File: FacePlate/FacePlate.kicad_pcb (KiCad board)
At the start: 4 copper layers, 131.1 x 44 mm, 76 parts, among them J2 GPIO, J3 Conn_01x04_Pin, U4 SX1280, U5 MCP2515-xST, U6 MCP2551-I-SN, U7 AMS1117-3.3, Y2 ABM3-8.000MHZ-D2Y-T

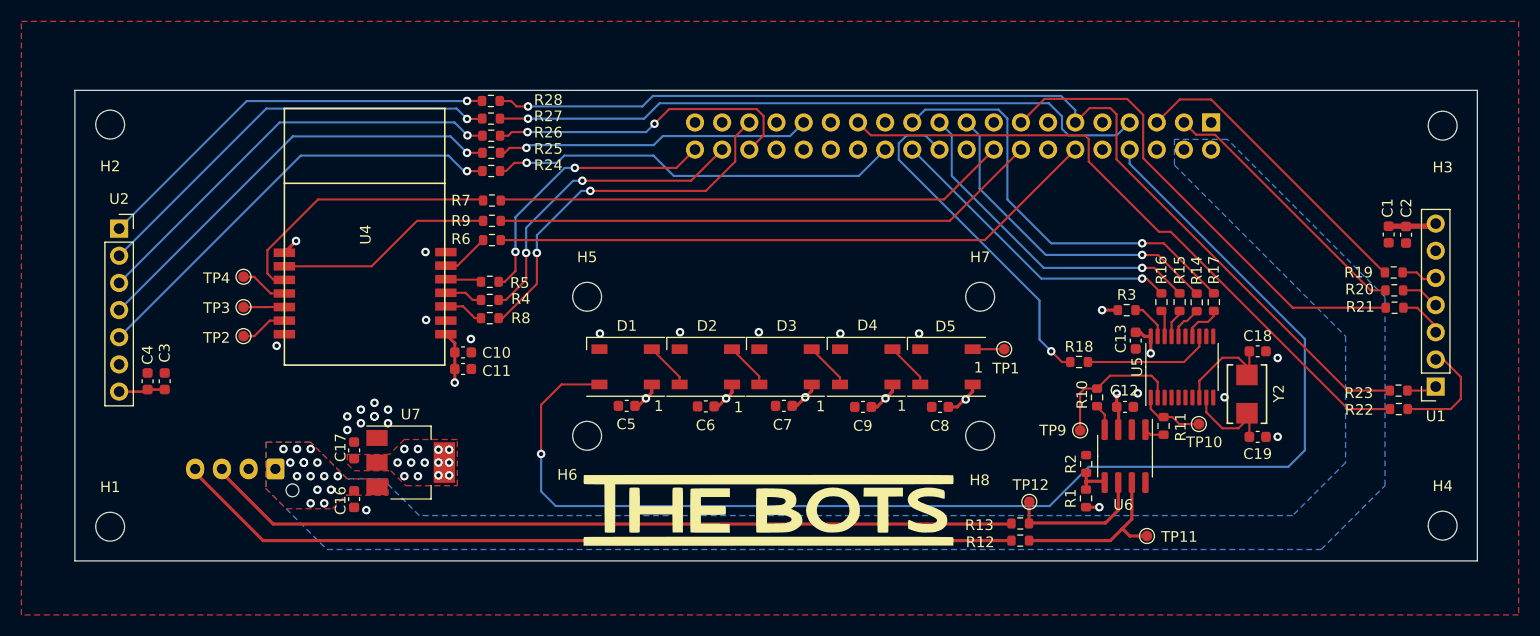
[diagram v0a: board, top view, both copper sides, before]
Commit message: faceplate updates
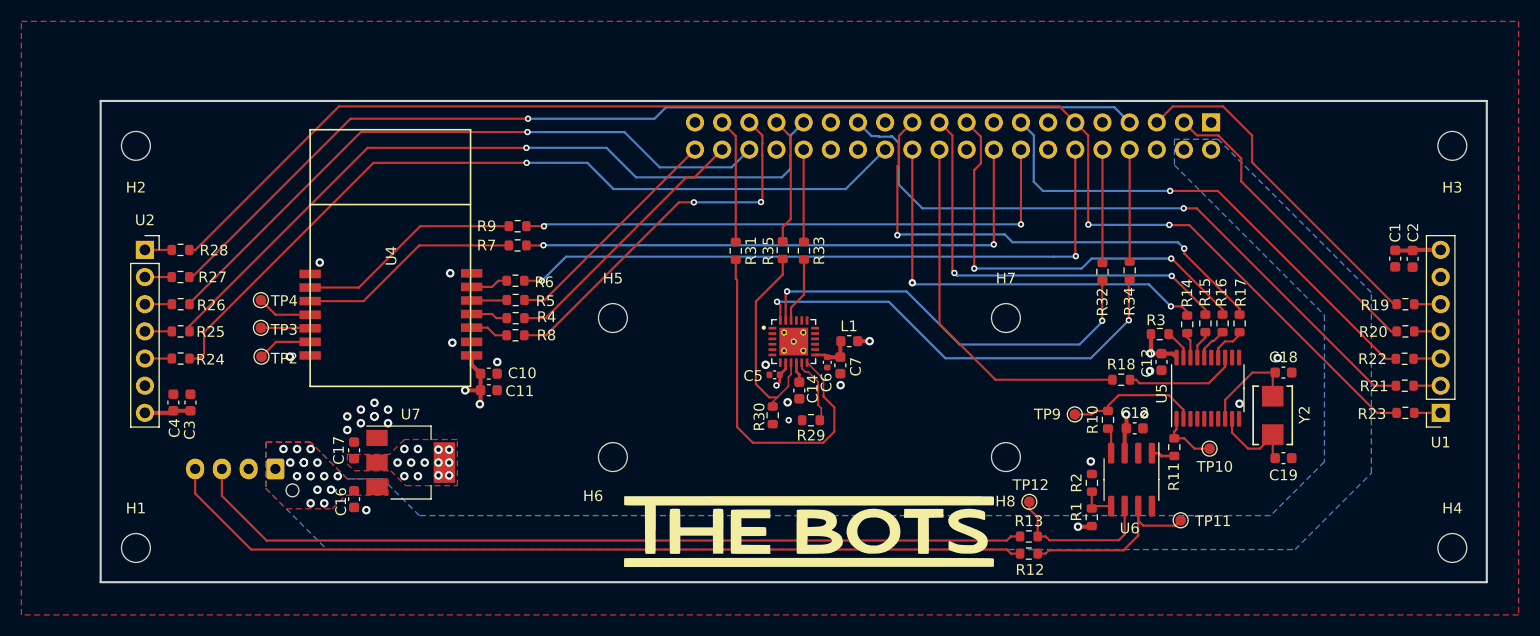
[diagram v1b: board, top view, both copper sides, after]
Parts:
- removed C8, C9: 100n, Capacitor_SMD:C_0603_1608Metric
- removed D1, D2, D3, D4, D5: WS2812B, LED_SMD:LED_WS2812B_PLCC4_5.0x5.0mm_P3.2mm
- removed TP1: TestPoint, TestPoint:TestPoint_Pad_D1.0mm
- added C14: 10u, bots:C_0603_1608Metric, F.Cu at (167.7, 84.1)
- added L1: 120R, bots:L_0603_1608Metric, F.Cu at (172.4, 79.5)
- added R29: 10k, bots:R_0603_1608Metric, F.Cu at (168.8, 86.8)
- added R30: 10k, bots:R_0603_1608Metric, F.Cu at (165.3, 86.4)
- added R31: 0R, bots:R_0603_1608Metric, F.Cu at (161.8, 71.0)
- added R32: 0R, bots:R_0603_1608Metric, F.Cu at (196.1, 73.0)
- added R33: 0R, bots:R_0603_1608Metric, F.Cu at (168.2, 71.0)
- added R34: 0R, bots:R_0603_1608Metric, F.Cu at (198.6, 72.8)
- added R35: 0R, bots:R_0603_1608Metric, F.Cu at (166.2, 70.9)
- added U3: ICM-20689, bots:QFN50P400X400X95-24N, F.Cu at (167.2, 79.5)
- C1, C10, C11, C2, C3, C4: value 100n -> 0.1u; footprint Capacitor_SMD:C_0603_1608Metric -> bots:C_0603_1608Metric
- C12, C13, C16: footprint Capacitor_SMD:C_0603_1608Metric -> bots:C_0603_1608Metric
- C17: value 22u -> 10u; footprint Capacitor_SMD:C_0603_1608Metric -> bots:C_0603_1608Metric
- C5, C6: footprint Capacitor_SMD:C_0603_1608Metric -> bots:C_0402_1005Metric
- C7: value 100n -> 10u; footprint Capacitor_SMD:C_0603_1608Metric -> bots:C_0603_1608Metric
- R10, R11, R12, R13, R14, R15, R16, R17, R18, R19, R20, R21, R22, R23, R24, R25, R26, R27, R28: value 0k -> 0R; footprint Resistor_SMD:R_0603_1608Metric -> bots:R_0603_1608Metric
- U1, U2: footprint Connector_PinSocket_2.54mm:PinSocket_1x07_P2.54mm_Vertical -> bots:GC9A_Display
- moved R24 33.9 mm to (109.9, 81.1)
- moved R25 33.5 mm to (109.9, 78.5)
- moved R26 33.0 mm to (109.9, 76.0)
- moved R27 32.6 mm to (109.9, 73.5)
- moved R28 32.2 mm to (109.9, 70.9)
- moved C5 14.1 mm to (165.4, 82.6)
- moved C6 12.1 mm to (170.4, 81.4), turned to -90 degrees
- moved R21 7.35 mm to (224.4, 83.6)
- moved C7 6.49 mm to (171.6, 81.7), turned to -90 degrees
- moved R16 6.05 mm to (207.3, 77.8)
- moved R7 4.84 mm to (141.4, 70.5)
- moved R22 4.73 mm to (224.3, 81.1)
- moved R6 4.39 mm to (141.2, 73.8)
- moved R18 4.28 mm to (197.8, 83.1)
- moved G*** 4.27 mm to (168.6, 97.2)
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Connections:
- C6 pad 1: +3.3V -> /IMU/3v3
- C7 pad 1: +3.3V -> /IMU/3v3
- R14 pad 1: Net-(U5-SI) -> Net-(U5-~{CS})
- R14 pad 2: /SPI0_MOSI -> /SPI0_NSS
- R16 pad 1: Net-(U5-~{CS}) -> Net-(U5-SI)
- R16 pad 2: /SPI0_NSS -> /SPI0_MOSI
- R21 pad 1: Net-(U1-DC) -> Net-(U1-CS)
- R21 pad 2: /GPIO[22] -> /SPI3_NSS
- R22 pad 1: Net-(U1-CS) -> Net-(U1-DC)
- R22 pad 2: /SPI3_NSS -> /GPIO[22]
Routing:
- net /SPI5_MOSI: track 123.4 -> 10.5 mm, vias 1 -> 0
- net /IMU/SDI: track 0.00 -> 42.3 mm, vias 0 -> 2
- net /SPI4_MOSI: track 29.7 -> 69.9 mm
- net Net-(U2-MOSI): track 41.7 -> 2.52 mm, vias 1 -> 0
- net /IMU/SCLK: track 0.00 -> 39.0 mm, vias 0 -> 2
- net Net-(U2-CLK): track 41.3 -> 2.52 mm, vias 1 -> 0
- net Net-(U2-DC): track 40.7 -> 2.52 mm, vias 1 -> 0
- net /SPI4_CLK: track 38.4 -> 76.3 mm
- net Net-(U2-CS): track 40.1 -> 2.51 mm, vias 1 -> 0
- net Net-(U2-RST): track 38.9 -> 2.51 mm, vias 1 -> 0
- net /GPIO[17]: track 99.5 -> 135.2 mm, vias 1 -> 2
- net /IMU/INT: track 0.00 -> 33.3 mm
- net /SPI4_NSS: track 61.9 -> 95.1 mm
- net /GPIO[16]: track 29.6 -> 61.1 mm, vias 2 -> 1
- net /IMU/SDO: track 0.00 -> 20.1 mm
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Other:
- board size 131.1 x 44 mm -> 129.6 x 45 mm
